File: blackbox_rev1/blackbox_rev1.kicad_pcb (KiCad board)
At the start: 2 copper layers, 83.8 x 53.3 mm, 17 parts, among them J1 RJ45_LED_Shielded, J2 Molex_uF_SV_06, J3 Conn_02x08_Counter_Clockwise, SW1 SW_Push, SW2 SW_Push, U1 Teensy4.1_DEV-16771, U2 TSR1-2433

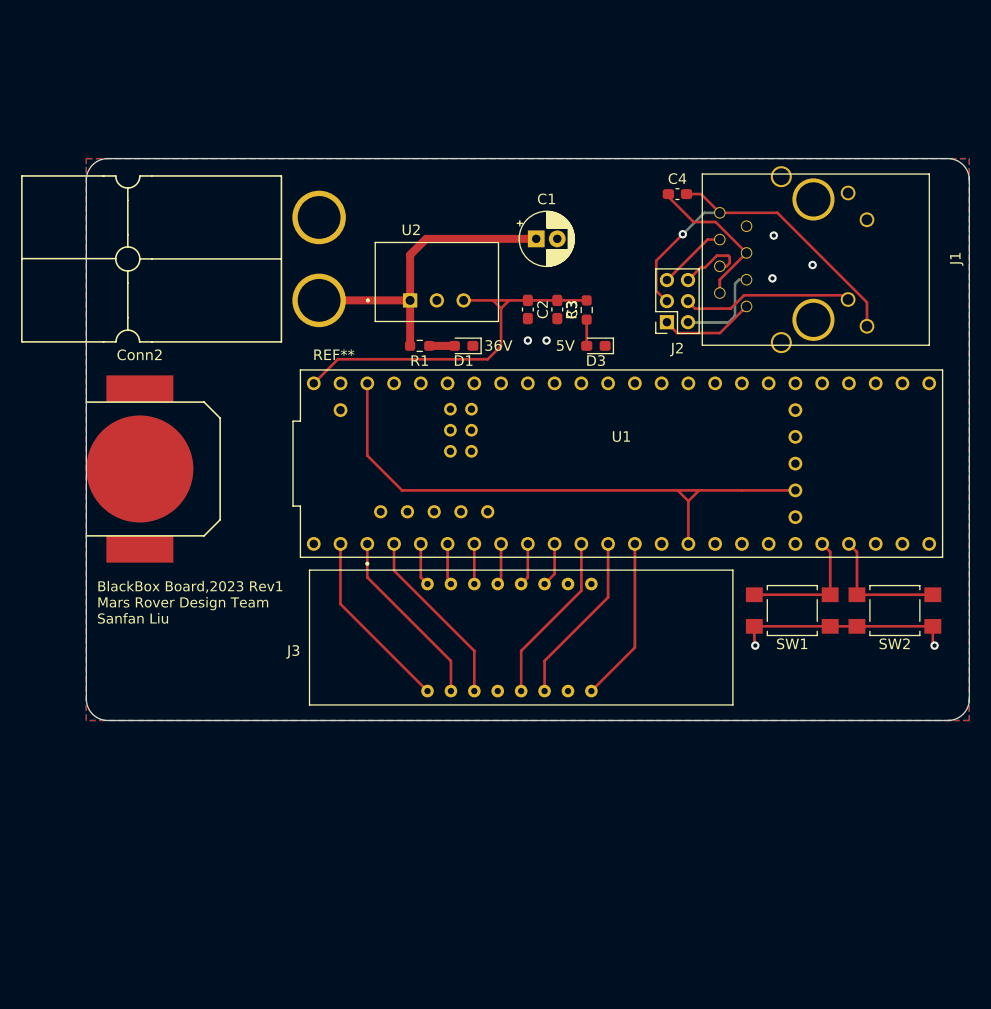
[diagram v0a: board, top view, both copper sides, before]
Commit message: hotfix
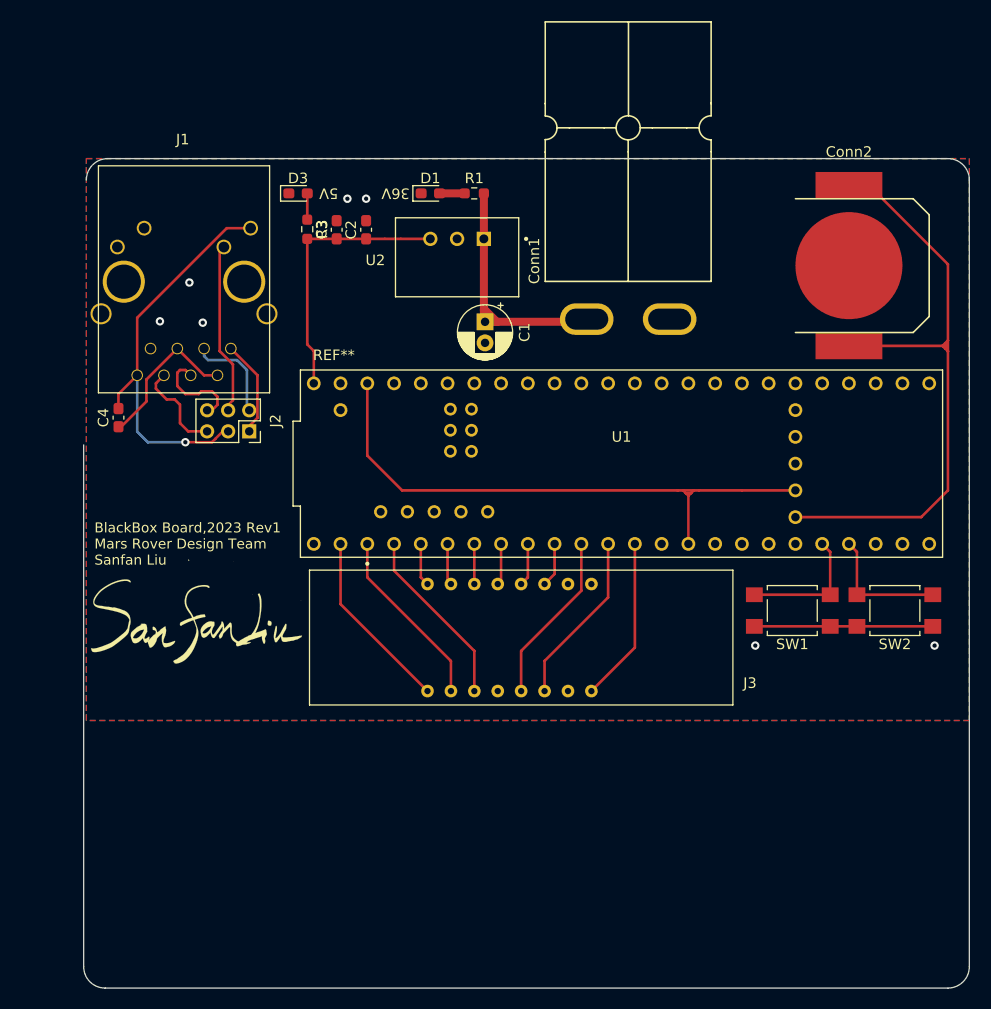
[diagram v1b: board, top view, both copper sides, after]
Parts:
- added G***: LOGO, MRDT_Silkscreens:z_sig_SanfanLiu_sig21.8mmx12.3mm1, F.Cu at (67.3, 96.3)
- Conn1: footprint MRDT_Connectors:Anderson_2_Horizontal_Side_by_Side -> MRDT_Connectors:Square_Anderson_2_H_Side_By_Side
- R1: value 3360 -> 2500
- R3: value 330 -> 200
- moved J1 73.7 mm to (66.3, 51.0), turned to 180 degrees
- moved Conn2 70.0 mm to (129.5, 54.9)
- moved C4 57.1 mm to (60.2, 76.9), turned to 90 degrees
- moved J2 41.0 mm to (72.6, 78.2), turned to -90 degrees
- moved Conn1 35.3 mm to (113.1, 67.9), turned to -90 degrees
- moved D3 31.8 mm to (77.2, 55.6), turned to 0 degrees
- moved R3 27.6 mm to (78.1, 59.0), turned to -90 degrees
- moved C3 22.3 mm to (80.9, 59.1), turned to 90 degrees
- moved C2 17.1 mm to (83.7, 59.1), turned to 90 degrees
- moved R1 15.4 mm to (94.0, 55.6), turned to 0 degrees
- moved D1 14.8 mm to (89.8, 55.6), turned to 0 degrees
- moved C1 9.25 mm to (95.0, 67.8), turned to -90 degrees
- moved U2 3.03 mm to (92.3, 61.7), turned to 180 degrees
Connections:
- net Net-(J1-Pad1) renamed /TX+
- net Net-(J1-Pad3) renamed /TX-
- net Net-(J1-Pad4) renamed /RX+
- net Net-(J1-Pad6) renamed /RX-
- Conn2 pad 1: (no net) -> VBAT
- Conn2 pad 2: (no net) -> GND
- U1 pad VBAT: Net-(Conn2-Pad+V) -> VBAT
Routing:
- net VBAT: track 0.00 -> 64.1 mm
- net +5V: track 36.6 -> 25.7 mm
- net +36V: track 29.9 -> 23.6 mm
- net GND: track 20.7 -> 17.3 mm
- net Net-(C4-Pad2): track 36.1 -> 38.6 mm
- net /RX-: track 6.64 -> 9.14 mm
- net /RX+: track 7.07 -> 9.26 mm
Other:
- board size 83.8 x 53.3 mm -> 84.1 x 78.7 mm
- board text added: "Keep Out Zone"
